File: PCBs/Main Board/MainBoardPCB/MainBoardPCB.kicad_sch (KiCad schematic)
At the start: 76 parts, among them J1 USB_B_Micro, J2 USB_B_Micro, J3 Conn_02x08_Odd_Even_MountingP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, J4 Conn_02x08_Odd_Even_MountingP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, J5 Conn_01x02, J6 Conn_01x02, J7 Conn_01x03, J8 Conn_01x03, U1 TPS566238PRQFR, U2 W25Q128JVS, U3 RP2040, U4 ESP32-S3-WROOM-1-N16, U5 MIC5219-3.3YM5, U6 MIC5219-3.3YM5, U7 LSM6DSVTR, Y1 ABM8-272-T3

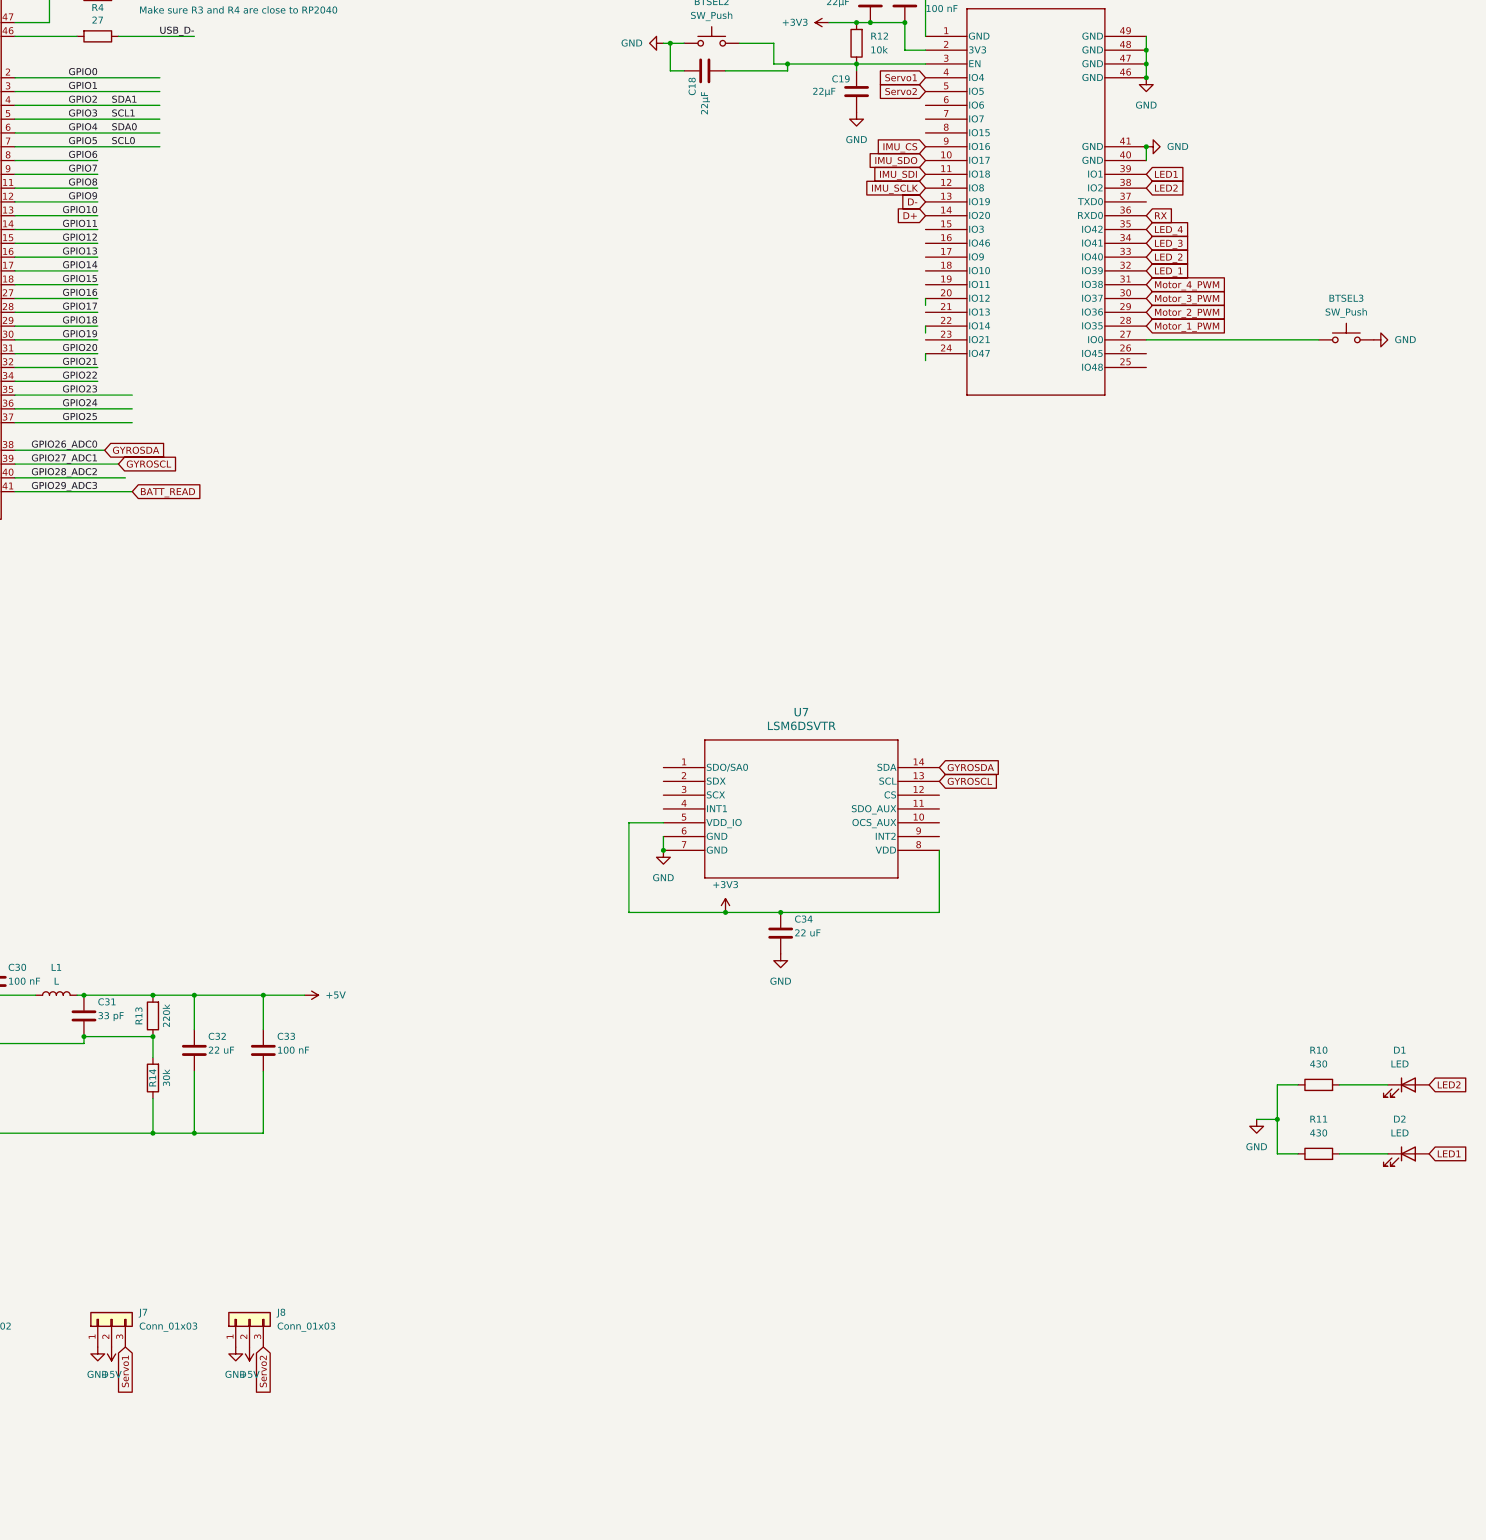
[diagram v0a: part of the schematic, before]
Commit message: Go us
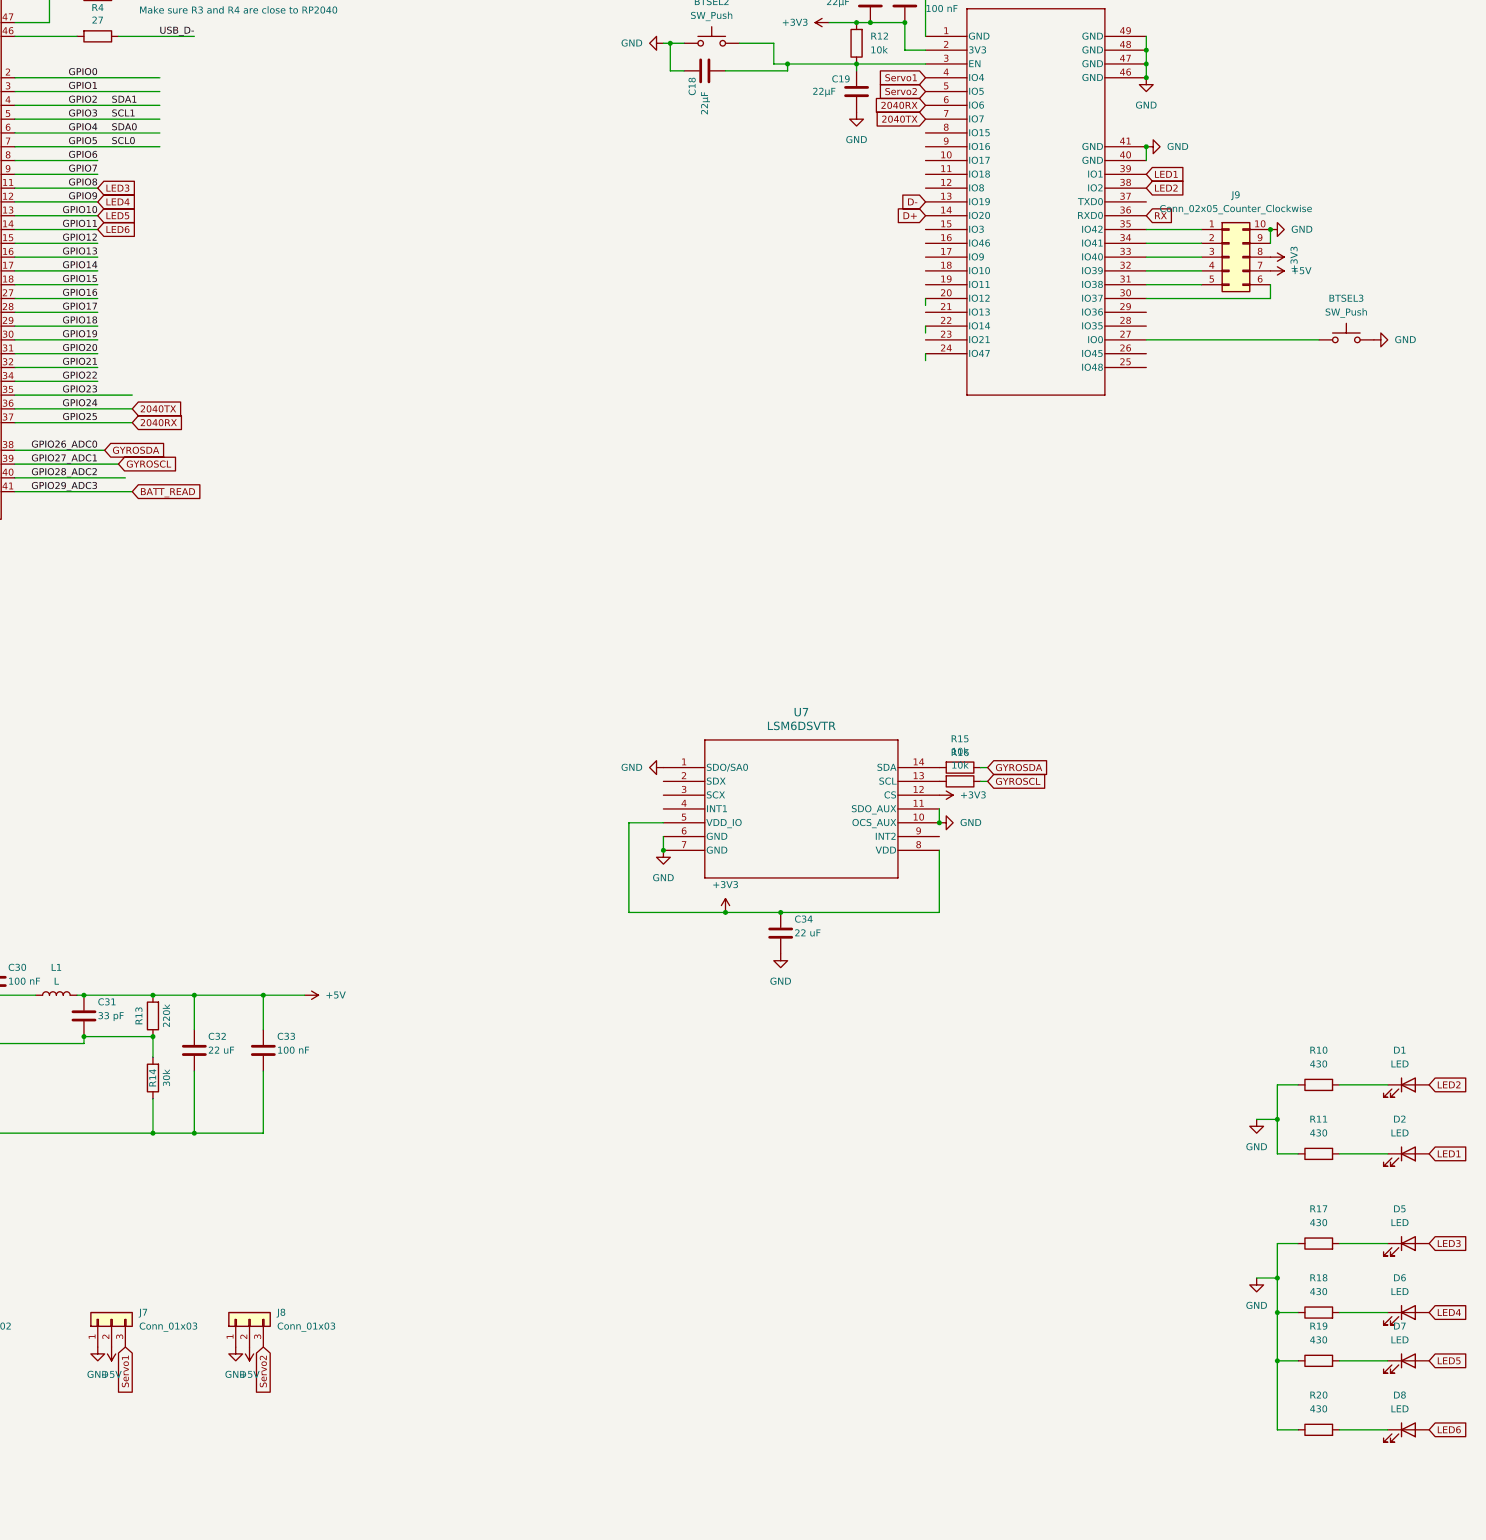
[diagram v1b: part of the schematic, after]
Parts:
- added D5, D6, D7, D8: LED, LED_SMD:LED_0603_1608Metric_Pad1.05x0.95mm_HandSolder, symbol Device:LED
- added J9: Conn_02x05_Counter_Clockwise, Connector_PinHeader_2.54mm:PinHeader_2x05_P2.54mm_Vertical, symbol Connector_Generic:Conn_02x05_Counter_Clockwise
- added R15, R16: 10k, Resistor_SMD:R_0402_1005Metric_Pad0.72x0.64mm_HandSolder, symbol Device:R
- added R17, R18, R19, R20: 430, Resistor_SMD:R_0402_1005Metric_Pad0.72x0.64mm_HandSolder, symbol Device:R
- D3, D4: footprint Diode_SMD:D_SOD-123F -> Diode_SMD:D_SOD-128
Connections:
- net GPIO24 is gone; now on net 2040TX: U3.36 (GPIO24)
- net GPIO25 is gone; now on net 2040RX: U3.37 (GPIO25)
- net +3V3: now also U7.12 (CS), J9.8 (Pin_8)
- net +5V: now also J9.7 (Pin_7)
- net GND: now also U7.1 (SDO/SA0), U7.10 (OCS_AUX), U7.11 (SDO_AUX), J9.10 (Pin_10), J9.9 (Pin_9), R17.1, R18.1, R19.1, R20.1
- net GYROSCL: now also R16.1; no longer U7.13 (SCL)
- net GYROSDA: now also R15.1; no longer U7.14 (SDA)
- net 2040RX: now reaches U4.6 (IO6)
- net 2040TX: now reaches U4.7 (IO7)
- net GPIO10 renamed LED5
- net LED5: now also D7.2 (A)
- net GPIO11 renamed LED6
- net LED6: now also D8.2 (A)
- net GPIO8 renamed LED3
- net LED3: now also D5.2 (A)
- net GPIO9 renamed LED4
- net LED4: now also D6.2 (A)
- net IMU_CS: no longer names the net of U4.9 (IO16)
- net IMU_SCLK: no longer names the net of U4.12 (IO8)
- net IMU_SDI: no longer names the net of U4.11 (IO18)
- net IMU_SDO: no longer names the net of U4.10 (IO17)
- net LED_1: no longer names the net of U4.32 (IO39)
- net LED_1: now also J9.4 (Pin_4)
- net LED_2: no longer names the net of U4.33 (IO40)
- net LED_2: now also J9.3 (Pin_3)
- net LED_3: no longer names the net of U4.34 (IO41)
- net LED_3: now also J9.2 (Pin_2)
- net LED_4: no longer names the net of U4.35 (IO42)
- net LED_4: now also J9.1 (Pin_1)
- net Motor_1_PWM: no longer names the net of U4.28 (IO35)
- net Motor_2_PWM: no longer names the net of U4.29 (IO36)
- net Motor_3_PWM: no longer names the net of U4.30 (IO37)
- net Motor_3_PWM: now also J9.6 (Pin_6)
- net Motor_4_PWM: no longer names the net of U4.31 (IO38)
- net Motor_4_PWM: now also J9.5 (Pin_5)
- new net: D7.1 (K), R19.2
- new net: R16.2, U7.13 (SCL)
- new net: R15.2, U7.14 (SDA)
- new net: D6.1 (K), R18.2
- new net: D5.1 (K), R17.2
- new net: D8.1 (K), R20.2

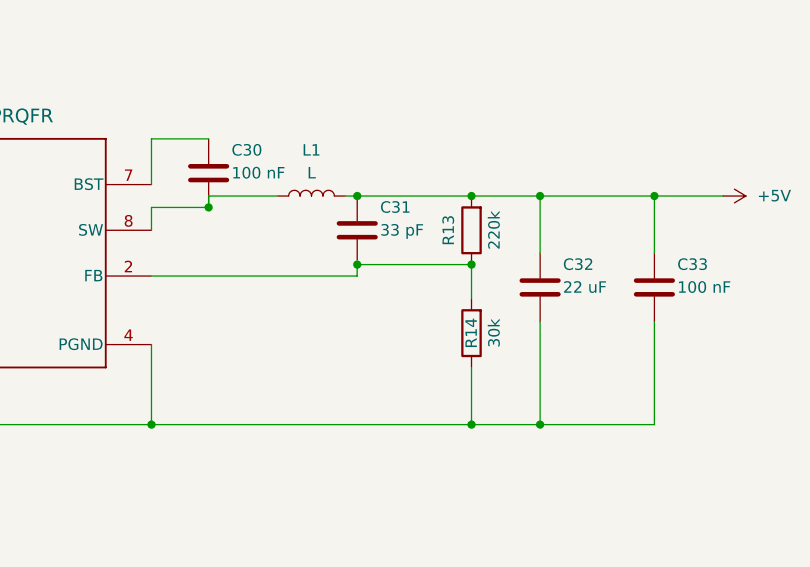
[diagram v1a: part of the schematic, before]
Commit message: vault backup: 2025-05-05 19:42:36
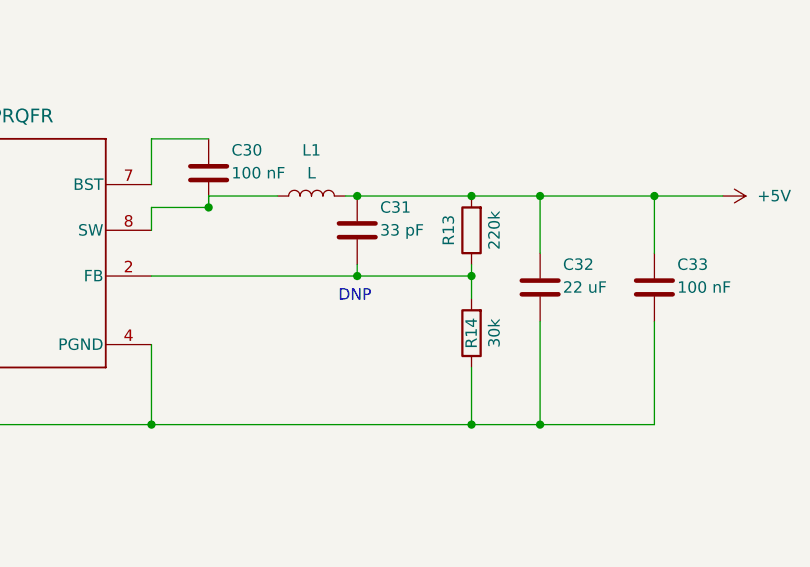
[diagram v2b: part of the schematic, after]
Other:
- note added: "DNP"
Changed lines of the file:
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@@
+		)
+	)
+	(text "DNP\n"
+		(exclude_from_sim no)
+		(at 221.996 252.476 0)
+		(effects
+			(font
+				(size 1.27 1.27)
+			)
 		)
 	)
@@
 	)
 	(junction
-		(at 234.95 248.92)
-		(diameter 0)
-		(color 0 0 0 0)
-	)
-	(junction
 		(at 24.13 307.34)
 		(diameter 0)
@@
 	)
 	(junction
-		(at 222.25 248.92)
-		(diameter 0)
-		(color 0 0 0 0)
-	)
-	(junction
 		(at 441.96 308.61)
 		(diameter 0)
@@
 	)
 	(junction
+		(at 222.25 250.19)
+		(diameter 0)
+		(color 0 0 0 0)
+	)
+	(junction
 		(at 271.78 33.02)
 		(diameter 0)
@@
 	(junction
 		(at 367.03 52.07)
+		(diameter 0)
+		(color 0 0 0 0)
+	)
+	(junction
+		(at 234.95 250.19)
 		(diameter 0)
 		(color 0 0 0 0)
@@
 	(wire
 		(pts
+			(xy 222.25 250.19) (xy 222.25 248.92)
+		)
+		(stroke
+			(width 0)
+			(type default)
+		)
+	)
+	(wire
+		(pts
 			(xy 199.39 234.95) (xy 199.39 240.03)
 		)
@@
 	(wire
 		(pts
+			(xy 234.95 250.19) (xy 234.95 252.73)
+		)
+		(stroke
+			(width 0)
+			(type default)
+		)
+	)
+	(wire
+		(pts
 			(xy 87.63 309.88) (xy 88.9 309.88)
 		)
@@
 	(wire
 		(pts
-			(xy 222.25 250.19) (xy 222.25 248.92)
-		)
-		(stroke
-			(width 0)
-			(type default)
-		)
-	)
-	(wire
-		(pts
 			(xy 26.67 48.26) (xy 24.13 48.26)
 		)
@@
 	(wire
 		(pts
-			(xy 222.25 248.92) (xy 234.95 248.92)
+			(xy 222.25 250.19) (xy 234.95 250.19)
 		)
 		(stroke
@@
 	(wire
 		(pts
-			(xy 234.95 248.92) (xy 234.95 252.73)
-		)
-		(stroke
+			(xy 234.95 248.92) (xy 234.95 250.19)
+		)
+		(stroke
